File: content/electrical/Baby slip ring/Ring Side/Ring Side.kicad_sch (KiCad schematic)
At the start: 6 parts, among them J1 USB4105-GF-A, U1 2_Wire_Ring

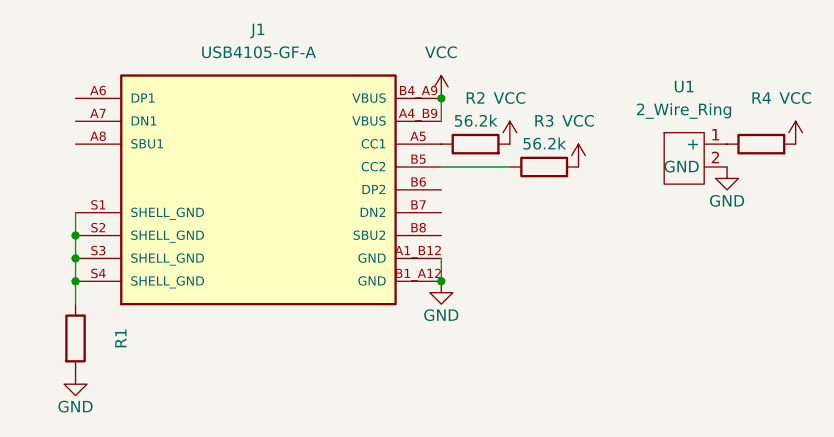
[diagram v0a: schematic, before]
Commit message: first save of babyslipring
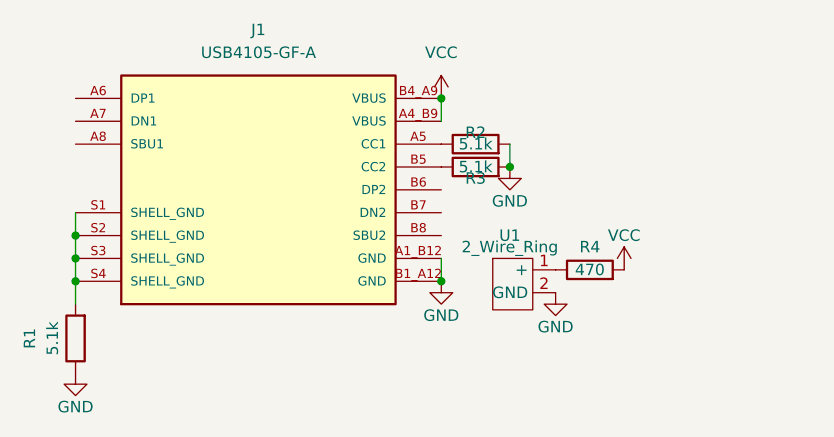
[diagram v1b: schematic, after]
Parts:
- R1: value (none) -> 5.1k; footprint (none) -> Resistor_SMD:R_0402_1005Metric
- R2, R3: value 56.2k -> 5.1k
- R4: value (none) -> 470; footprint (none) -> Resistor_SMD:R_0402_1005Metric
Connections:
- net GND: now also R1.1, R2.2, R3.2; no longer R1.2
- net VCC: no longer R2.2, R3.2
- net at J1.S1 (SHELL_GND), J1.S2 (SHELL_GND), J1.S3 (SHELL_GND)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: now also R1.2; no longer R1.1
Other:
- moved on the sheet: R4, U1
